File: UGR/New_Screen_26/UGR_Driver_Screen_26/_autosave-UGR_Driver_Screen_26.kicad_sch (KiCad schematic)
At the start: 57 parts, among them J1 Conn_01x04, J2 Conn_01x40_Socket, J5 USB_B_Micro, SW1 SW_Nidec_CAS-120A1, SW2 SW_Push, U2 STM32F405VGTx, U3 MCP2562-E-MF, U4 TPS562200, U5 TPS562200

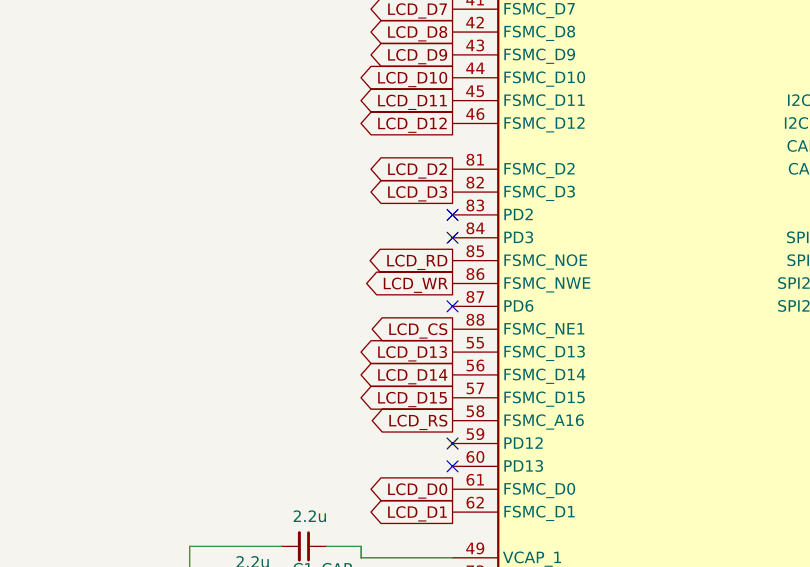
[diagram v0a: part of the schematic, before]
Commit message: Comms 3 + Rover
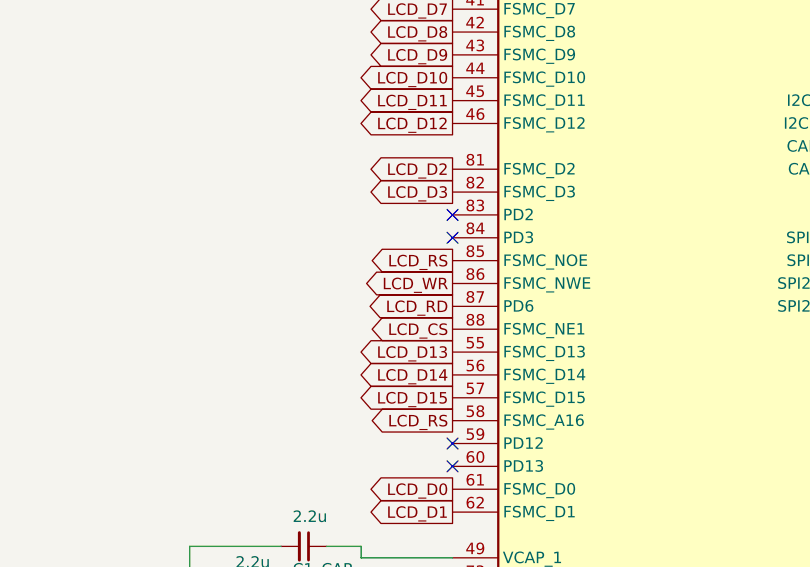
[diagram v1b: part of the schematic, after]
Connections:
- net LCD_RD: now also U2.87 (PD6); no longer U2.85 (PD4)
- net LCD_RS: now also U2.85 (PD4)
- no-connect marks 53 -> 52
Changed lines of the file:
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@@
 	)
 	(no_connect
-		(at 67.31 214.63)
-	)
-	(no_connect
 		(at 214.63 237.49)
 	)
@@
 		)
 	)
+	(global_label "LCD_RD"
+		(shape output)
+		(at 67.31 214.63 180)
+		(fields_autoplaced yes)
+		(effects
+			(font
+				(size 1.27 1.27)
+			)
+			(justify right)
+		)
+		(property "Intersheetrefs" "${INTERSHEET_REFS}"
+			(at 57.2491 214.63 0)
+			(effects
+				(font
+					(size 1.27 1.27)
+				)
+				(justify right)
+				(hide yes)
+			)
+		)
+	)
 	(global_label "SD_MISO"
 		(shape output)
@@
 		)
 	)
-	(global_label "LCD_RD"
+	(global_label "LCD_RS"
 		(shape output)
 		(at 67.31 209.55 180)
@@
 		)
 		(property "Intersheetrefs" "${INTERSHEET_REFS}"
-			(at 57.2491 209.55 0)
+			(at 57.3096 209.55 0)
 			(effects
 				(font
